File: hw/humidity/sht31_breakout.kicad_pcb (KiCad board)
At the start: 2 copper layers, 20.6 x 6.6 mm, 6 parts, among them P1 CONN_01X03, P2 CONN_01X03, U1 SHT3x-DIS

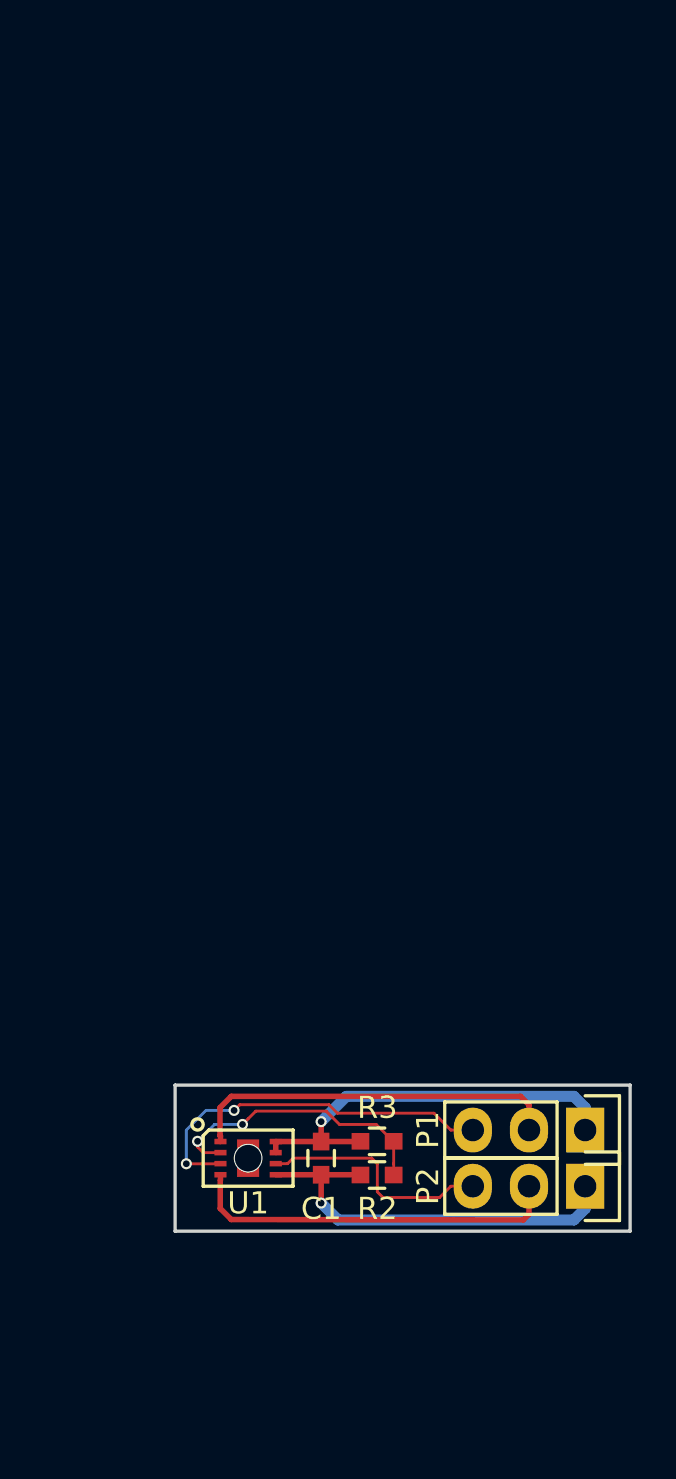
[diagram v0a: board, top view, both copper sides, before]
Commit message: Start designing flex pcb :D
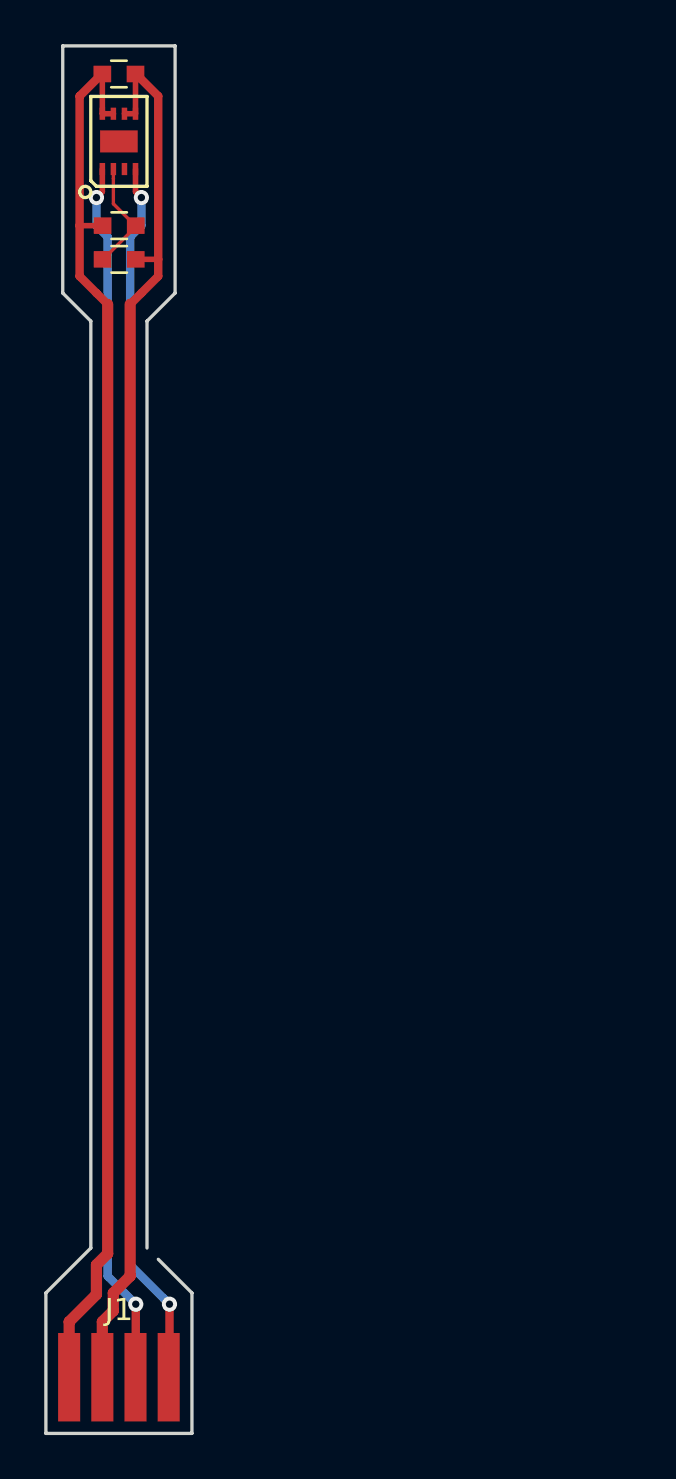
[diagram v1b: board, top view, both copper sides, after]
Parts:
- removed P1, P2: CONN_01X03, Pin_Headers:Pin_Header_Straight_1x03
- added J1: CONN_01X04, footprints:smd_flex_4, F.Cu at (139.7, 124.5)
- moved C1 49.9 mm to (139.7, 65.5), turned to 180 degrees
- moved U1 46.3 mm to (139.7, 68.6), turned to 90 degrees
- moved R2 43.0 mm to (139.7, 73.9), turned to 180 degrees
- moved R3 43.0 mm to (139.7, 72.4)
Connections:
- U1 pad 3: /ALERT -> Net-(U1-Pad3)
- U1 pad 6: /nRESET -> VDD
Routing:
- net VDD: track 18.6 -> 63.7 mm, vias 1 -> 0
- net GND: track 18.9 -> 64.0 mm, vias 1 -> 0
- net /SCL: track 17.1 -> 55.7 mm, vias 0 -> 2
- net /SDA: track 17.0 -> 55.5 mm, vias 0 -> 2
- net /ALERT: track 17.0 -> 0.00 mm, vias 2 -> 0
- net /nRESET: track 10.7 -> 0.00 mm
- net /ADDR: track 12.9 -> 5.15 mm, vias 2 -> 0
- net (no net): vias 1 -> 0
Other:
- board size 20.6 x 6.6 mm -> 6.6 x 62.7 mm
- net class Default: clearance 0.16 -> 0.1524; trace_width 0.13 -> 0.1524; via_dia 0.5 -> 0.6858; via_drill 0.305 -> 0.3302
- rule trace_clearance: 0.16 -> 0.1524
- rule trace_min: 0.13 -> 0.1524
- rule via_min_drill: 0.305 -> 0.3302
- rule via_min_size: 0.5 -> 0.6858
- board text removed: "@alvaroprieto"
- board text removed: "ostur humidity 1.1"
